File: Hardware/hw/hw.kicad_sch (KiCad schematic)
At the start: 0 parts

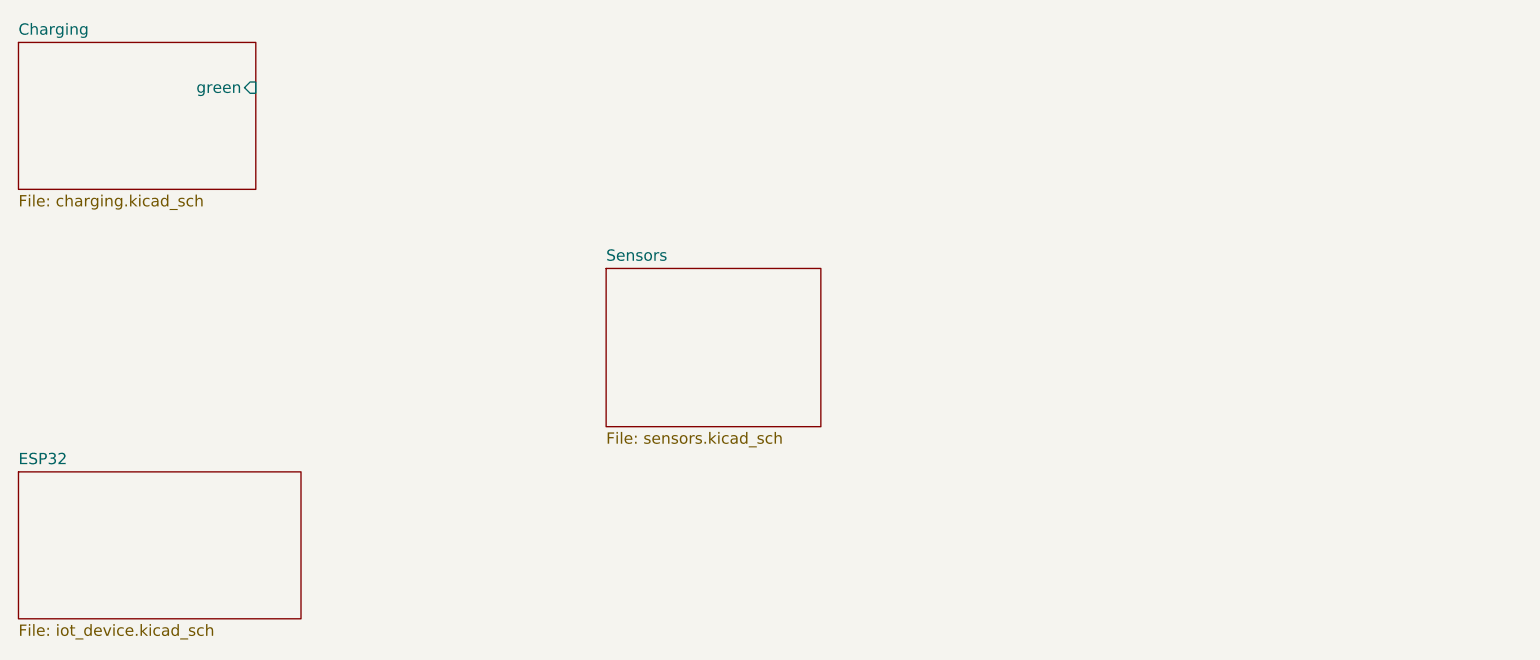
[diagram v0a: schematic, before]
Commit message: Hardware v1.0
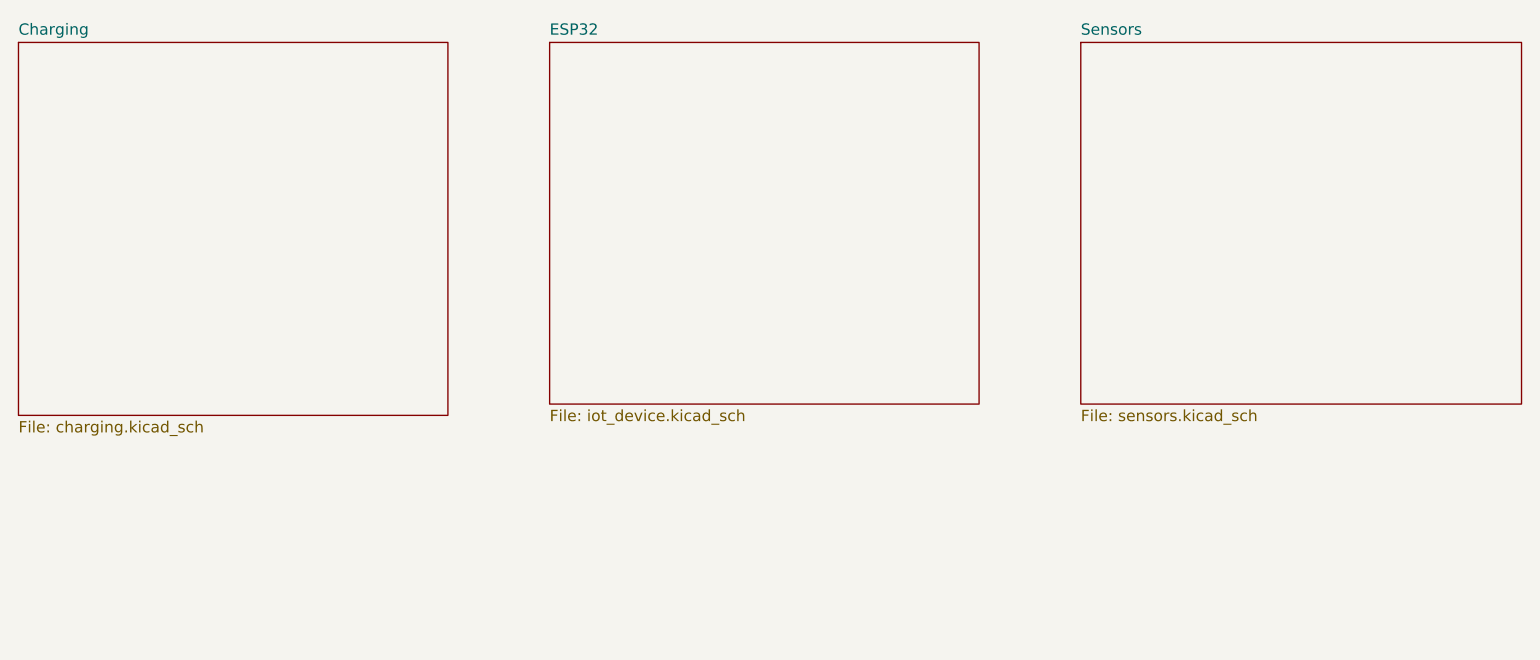
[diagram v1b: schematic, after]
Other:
- sheet Charging ports: added none; removed green
- company: (none) -> UNIZA Faculty of Management Science and Informatics Department of Technical Cybernetics
- title: (none) -> Solar Power Management and Monitoring Circuit
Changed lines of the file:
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@@
 	(generator_version "9.0")
 	(paper "A4")
+	(title_block
+		(title "Solar Power Management and Monitoring Circuit")
+		(date "2026-04-24")
+		(rev "Tomáš Bača")
+		(company "UNIZA Faculty of Management Science and Informatics Department of Technical Cybernetics")
+		(comment 1 "Author: Peter Kolok")
+	)
 	(sheet
-		(at 44.45 66.04)
-		(size 31.75 16.51)
+		(at 104.14 17.78)
+		(size 48.26 40.64)
 		(exclude_from_sim no)
 		(in_bom yes)
@@
 		)
 		(property "Sheetname" "ESP32"
-			(at 44.45 65.3284 0)
+			(at 104.14 17.0684 0)
 			(effects
 				(font
@@
 		)
 		(property "Sheetfile" "iot_device.kicad_sch"
-			(at 44.45 83.1346 0)
+			(at 104.14 59.0046 0)
 			(effects
 				(font
@@
 	(sheet
 		(at 44.45 17.78)
-		(size 26.67 16.51)
+		(size 48.26 41.91)
 		(exclude_from_sim no)
 		(in_bom yes)
@@
 		)
 		(property "Sheetfile" "charging.kicad_sch"
-			(at 44.45 34.8746 0)
+			(at 44.45 60.2746 0)
 			(effects
 				(font
@@
 				)
 				(justify left top)
-			)
-		)
-		(pin "green" input
-			(at 71.12 22.86 0)
-			(effects
-				(font
-					(size 1.27 1.27)
-				)
-				(justify right)
 			)
 		)
@@
 	)
 	(sheet
-		(at 110.49 43.18)
-		(size 24.13 17.78)
+		(at 163.83 17.78)
+		(size 49.53 40.64)
 		(exclude_from_sim no)
 		(in_bom yes)
@@
 		)
 		(property "Sheetname" "Sensors"
-			(at 110.49 42.4684 0)
+			(at 163.83 17.0684 0)
 			(effects
 				(font
@@
 		)
 		(property "Sheetfile" "sensors.kicad_sch"
-			(at 110.49 61.5446 0)
+			(at 163.83 59.0046 0)
 			(effects
 				(font
